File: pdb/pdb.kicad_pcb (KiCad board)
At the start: 2 copper layers, 50.8 x 76.2 mm, 25 parts, among them J1 Conn_01x02, U1 INA169, U2 LM7812_TO220, U3 NCP1117-5.0_TO252

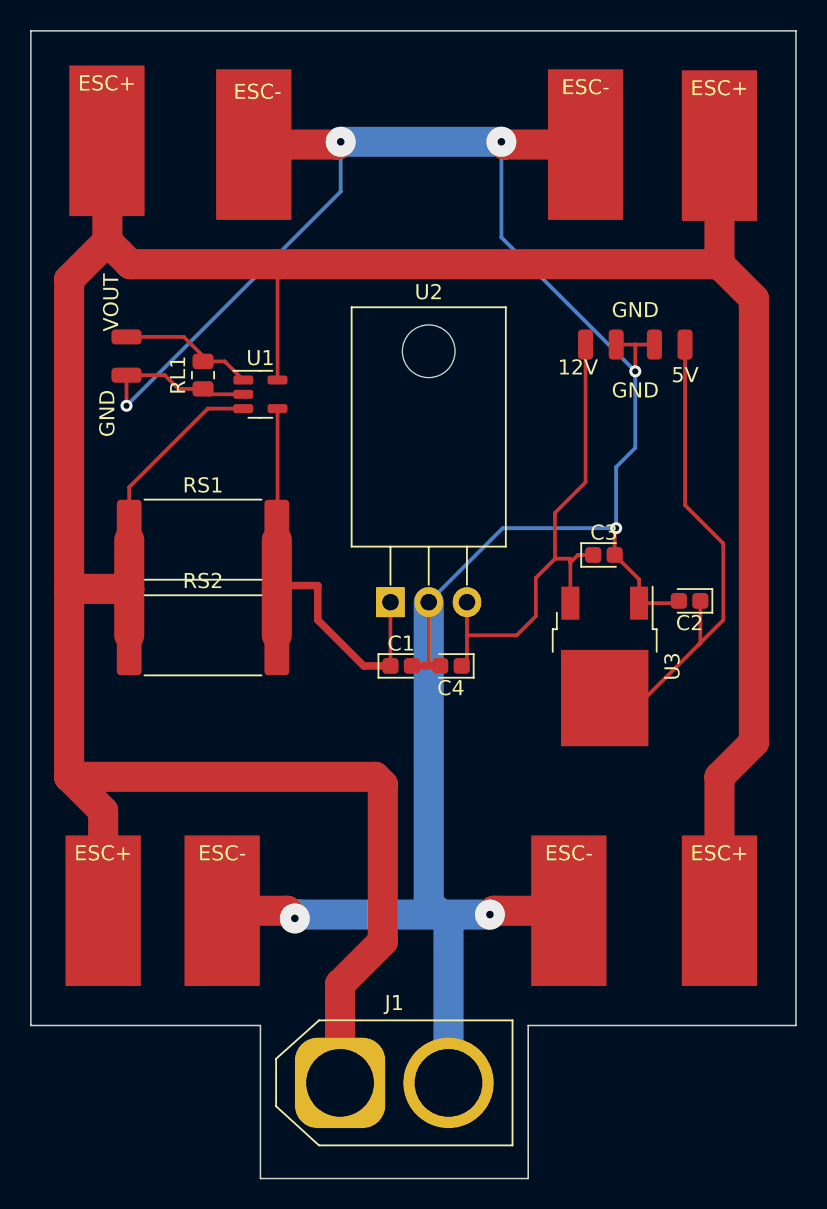
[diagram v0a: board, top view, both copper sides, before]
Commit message: updated files
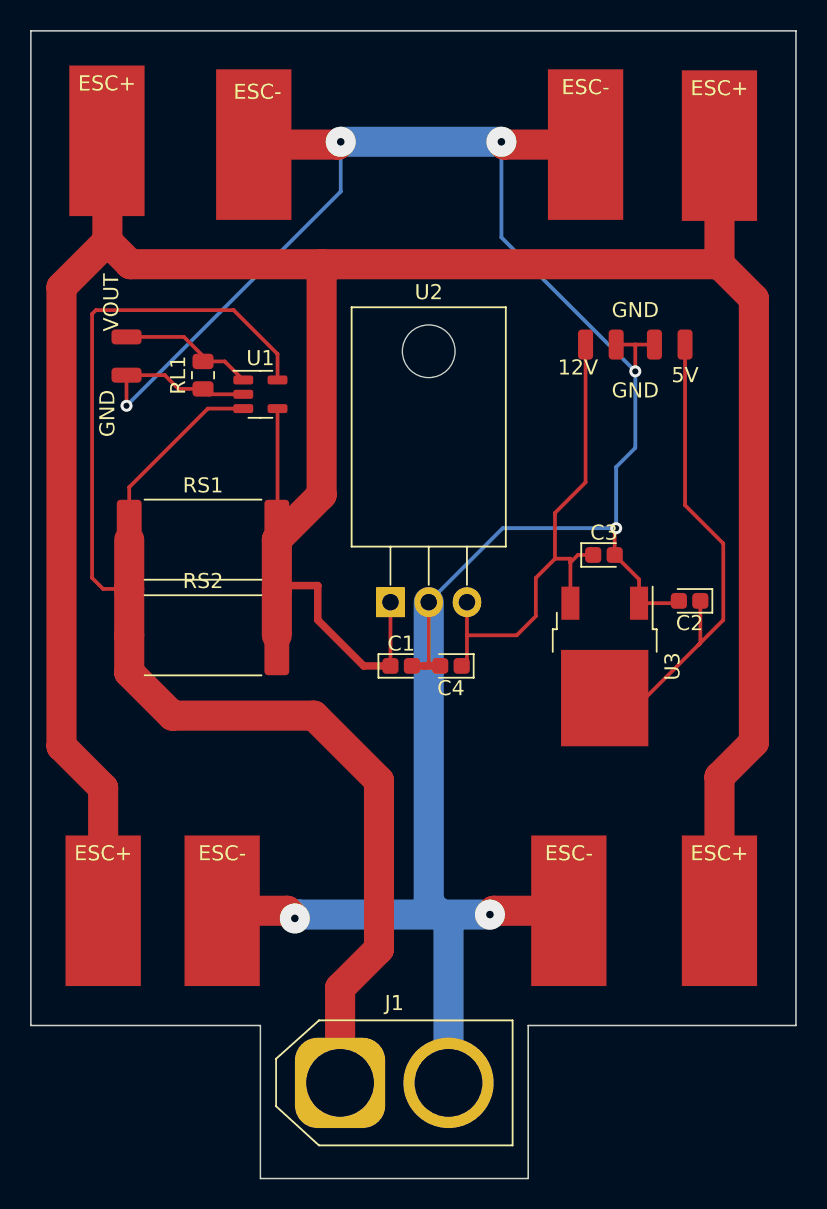
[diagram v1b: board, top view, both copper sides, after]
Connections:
- ESC+ pad 1: Net-(J1-Pad1) -> Net-(RS1-Pad2) (x4)
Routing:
- net Net-(RS1-Pad2): track 30.5 -> 197.6 mm
- net Net-(J1-Pad1): track 220.4 -> 98.4 mm
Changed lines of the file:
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@@
     (fp_line (start 2.75 -5.25) (end -2.75 -5.25) (layer "F.CrtYd") (width 0.05))
     (pad "1" smd rect (at 0 0) (size 5 10) (layers "F.Cu" "F.Paste" "F.Mask")
-      (net 5 "Net-(J1-Pad1)"))
+      (net 1 "Net-(RS1-Pad2)"))
   )
   (footprint "Capacitor_Tantalum_SMD:CP_EIA-1608-10_AVX-L" (layer "F.Cu")
@@
     (fp_line (start -2.75 5.25) (end 2.75 5.25) (layer "F.CrtYd") (width 0.05))
     (pad "1" smd rect (at 0 0) (size 5 10) (layers "F.Cu" "F.Paste" "F.Mask")
-      (net 5 "Net-(J1-Pad1)"))
+      (net 1 "Net-(RS1-Pad2)"))
   )
   (footprint "Resistor_SMD:R_4020_10251Metric_Pad1.65x5.30mm_HandSolder" (layer "F.Cu")
@@
     (fp_line (start -2.75 -5.25) (end -2.75 5.25) (layer "F.CrtYd") (width 0.05))
     (pad "1" smd rect (at 0 0) (size 5 10) (layers "F.Cu" "F.Paste" "F.Mask")
-      (net 5 "Net-(J1-Pad1)"))
+      (net 1 "Net-(RS1-Pad2)"))
   )
   (footprint "Connector_Wire:SolderWirePad_1x01_SMD_5x10mm" (layer "F.Cu")
@@
     (fp_line (start 2.75 -5.25) (end -2.75 -5.25) (layer "F.CrtYd") (width 0.05))
     (pad "1" smd rect (at 0 0) (size 5 10) (layers "F.Cu" "F.Paste" "F.Mask")
-      (net 5 "Net-(J1-Pad1)"))
+      (net 1 "Net-(RS1-Pad2)"))
   )
   (footprint "Connector_Wire:SolderWirePad_1x01_SMD_1x2mm" (layer "F.Cu")
@@
   (gr_line (start 12.7 12.7) (end 63.5 12.7) (layer "Margin") (width 0.15))
   (gr_line (start 27.94 78.74) (end 12.7 78.74) (layer "Margin") (width 0.15))
+  (segment (start 17.5 71.12) (end 17.5 62.966) (width 2) (layer "F.Cu") (net 1))
+  (segment (start 32.004 28.194) (end 58.42 28.194) (width 2) (layer "F.Cu") (net 1))
+  (segment (start 32.004 43.508) (end 29.03 46.482) (width 2) (layer "F.Cu") (net 1))
+  (segment (start 58.42 20.32) (end 58.42 28.194) (width 2) (layer "F.Cu") (net 1))
   (segment (start 36.576 54.864) (end 34.798 54.864) (width 0.5) (layer "F.Cu") (net 1))
   (segment (start 29.03 49.858) (end 29.03 52.832) (width 2) (layer "F.Cu") (net 1))
   (segment (start 29.0775 46.4345) (end 29.03 46.482) (width 0.25) (layer "F.Cu") (net 1))
   (segment (start 29.03 46.482) (end 29.03 49.858) (width 2) (layer "F.Cu") (net 1))
+  (segment (start 58.42 71.12) (end 58.42 62.23) (width 2) (layer "F.Cu") (net 1))
   (segment (start 34.798 54.864) (end 31.75 51.816) (width 0.5) (layer "F.Cu") (net 1))
+  (segment (start 14.732 60.198) (end 14.732 29.718) (width 2) (layer "F.Cu") (net 1))
   (segment (start 36.576 50.632) (end 36.576 54.864) (width 0.25) (layer "F.Cu") (net 1))
+  (segment (start 60.706 59.944) (end 58.42 62.23) (width 2) (layer "F.Cu") (net 1))
   (segment (start 29.0775 37.78) (end 29.0775 46.4345) (width 0.25) (layer "F.Cu") (net 1))
+  (segment (start 17.78 26.67) (end 17.78 20.03) (width 2) (layer "F.Cu") (net 1))
   (segment (start 31.75 51.816) (end 31.75 49.53) (width 0.5) (layer "F.Cu") (net 1))
+  (segment (start 17.5 62.966) (end 14.732 60.198) (width 2) (layer "F.Cu") (net 1))
+  (segment (start 14.732 29.718) (end 17.78 26.67) (width 2) (layer "F.Cu") (net 1))
+  (segment (start 60.706 30.48) (end 60.706 59.944) (width 2) (layer "F.Cu") (net 1))
+  (segment (start 19.304 28.194) (end 17.78 26.67) (width 2) (layer "F.Cu") (net 1))
+  (segment (start 32.004 28.194) (end 32.004 43.508) (width 2) (layer "F.Cu") (net 1))
+  (segment (start 19.304 28.194) (end 32.004 28.194) (width 2) (layer "F.Cu") (net 1))
   (segment (start 31.75 49.53) (end 29.358 49.53) (width 0.5) (layer "F.Cu") (net 1))
   (segment (start 29.358 49.53) (end 29.03 49.858) (width 0.5) (layer "F.Cu") (net 1))
+  (segment (start 17.78 20.03) (end 17.75 20) (width 2) (layer "F.Cu") (net 1))
+  (segment (start 58.42 28.194) (end 60.706 30.48) (width 2) (layer "F.Cu") (net 1))
   (segment (start 22.5025 36.4725) (end 21.59 35.56) (width 0.25) (layer "F.Cu") (net 2))
   (segment (start 39.116 54.61) (end 38.862 54.864) (width 0.25) (layer "F.Cu") (net 2))
@@
   (segment (start 48.521 50.699) (end 48.521 47.999) (width 0.25) (layer "F.Cu") (net 4))
   (segment (start 47.498 44.704) (end 47.498 47.738) (width 0.25) (layer "F.Cu") (net 4))
-  (segment (start 29.21 28.194) (end 19.304 28.194) (width 2) (layer "F.Cu") (net 5))
-  (segment (start 17.5 71.12) (end 17.5 64.49) (width 2) (layer "F.Cu") (net 5))
-  (segment (start 58.42 20.32) (end 58.42 28.194) (width 2) (layer "F.Cu") (net 5))
-  (segment (start 36.068 73.152) (end 36.068 62.738) (width 2) (layer "F.Cu") (net 5))
+  (segment (start 29.0775 34.1575) (end 26.162 31.242) (width 0.25) (layer "F.Cu") (net 5))
+  (segment (start 16.764 49.022) (end 17.494 49.752) (width 0.25) (layer "F.Cu") (net 5))
   (segment (start 19.23 49.752) (end 19.23 52.832) (width 2) (layer "F.Cu") (net 5))
-  (segment (start 19.23 49.752) (end 15.272 49.752) (width 2) (layer "F.Cu") (net 5))
-  (segment (start 15.24 49.784) (end 15.24 29.21) (width 2) (layer "F.Cu") (net 5))
-  (segment (start 58.42 71.12) (end 58.42 62.23) (width 2) (layer "F.Cu") (net 5))
-  (segment (start 35.56 62.23) (end 15.24 62.23) (width 2) (layer "F.Cu") (net 5))
-  (segment (start 60.706 59.944) (end 58.42 62.23) (width 2) (layer "F.Cu") (net 5))
-  (segment (start 58.42 28.194) (end 29.21 28.194) (width 2) (layer "F.Cu") (net 5))
-  (segment (start 33.23 82.55) (end 33.23 75.99) (width 2) (layer "F.Cu") (net 5))
-  (segment (start 15.24 29.21) (end 17.78 26.67) (width 2) (layer "F.Cu") (net 5))
+  (segment (start 33.23 76.244) (end 35.814 73.66) (width 2) (layer "F.Cu") (net 5))
+  (segment (start 31.496 58.166) (end 22.098 58.166) (width 2) (layer "F.Cu") (net 5))
+  (segment (start 16.764 31.496) (end 16.764 49.022) (width 0.25) (layer "F.Cu") (net 5))
+  (segment (start 35.814 62.484) (end 31.496 58.166) (width 2) (layer "F.Cu") (net 5))
   (segment (start 26.8025 37.78) (end 24.45 37.78) (width 0.25) (layer "F.Cu") (net 5))
-  (segment (start 36.068 62.738) (end 35.56 62.23) (width 2) (layer "F.Cu") (net 5))
-  (segment (start 17.78 26.67) (end 17.78 20.03) (width 2) (layer "F.Cu") (net 5))
-  (segment (start 29.0775 35.88) (end 29.0775 28.3265) (width 0.25) (layer "F.Cu") (net 5))
-  (segment (start 60.706 30.48) (end 60.706 59.944) (width 2) (layer "F.Cu") (net 5))
+  (segment (start 26.162 31.242) (end 17.018 31.242) (width 0.25) (layer "F.Cu") (net 5))
+  (segment (start 33.23 82.55) (end 33.23 76.244) (width 2) (layer "F.Cu") (net 5))
   (segment (start 19.23 46.482) (end 19.23 49.752) (width 2) (layer "F.Cu") (net 5))
-  (segment (start 33.23 75.99) (end 36.068 73.152) (width 2) (layer "F.Cu") (net 5))
-  (segment (start 19.304 28.194) (end 17.78 26.67) (width 2) (layer "F.Cu") (net 5))
-  (segment (start 15.24 62.23) (end 15.24 49.784) (width 2) (layer "F.Cu") (net 5))
-  (segment (start 29.0775 28.3265) (end 29.21 28.194) (width 0.25) (layer "F.Cu") (net 5))
+  (segment (start 22.098 58.166) (end 19.23 55.298) (width 2) (layer "F.Cu") (net 5))
+  (segment (start 17.018 31.242) (end 16.764 31.496) (width 0.25) (layer "F.Cu") (net 5))
   (segment (start 24.45 37.78) (end 19.23 43) (width 0.25) (layer "F.Cu") (net 5))
   (segment (start 19.23 43) (end 19.23 46.482) (width 0.25) (layer "F.Cu") (net 5))
-  (segment (start 15.272 49.752) (end 15.24 49.784) (width 2) (layer "F.Cu") (net 5))
-  (segment (start 17.78 20.03) (end 17.75 20) (width 2) (layer "F.Cu") (net 5))
-  (segment (start 17.5 64.49) (end 15.24 62.23) (width 2) (layer "F.Cu") (net 5))
-  (segment (start 58.42 28.194) (end 60.706 30.48) (width 2) (layer "F.Cu") (net 5))
+  (segment (start 19.23 55.298) (end 19.23 52.832) (width 2) (layer "F.Cu") (net 5))
+  (segment (start 17.494 49.752) (end 19.23 49.752) (width 0.25) (layer "F.Cu") (net 5))
+  (segment (start 35.814 73.66) (end 35.814 62.484) (width 2) (layer "F.Cu") (net 5))
+  (segment (start 29.0775 35.88) (end 29.0775 34.1575) (width 0.25) (layer "F.Cu") (net 5))
   (segment (start 25.57 34.6475) (end 24.13 34.6475) (width 0.25) (layer "F.Cu") (net 6))
   (segment (start 24.13 34.6475) (end 24.13 34.29) (width 0.25) (layer "F.Cu") (net 6))
